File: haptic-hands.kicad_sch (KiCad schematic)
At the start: 17 parts, among them M1 Motor_DC, SW1 SW_Push_45deg

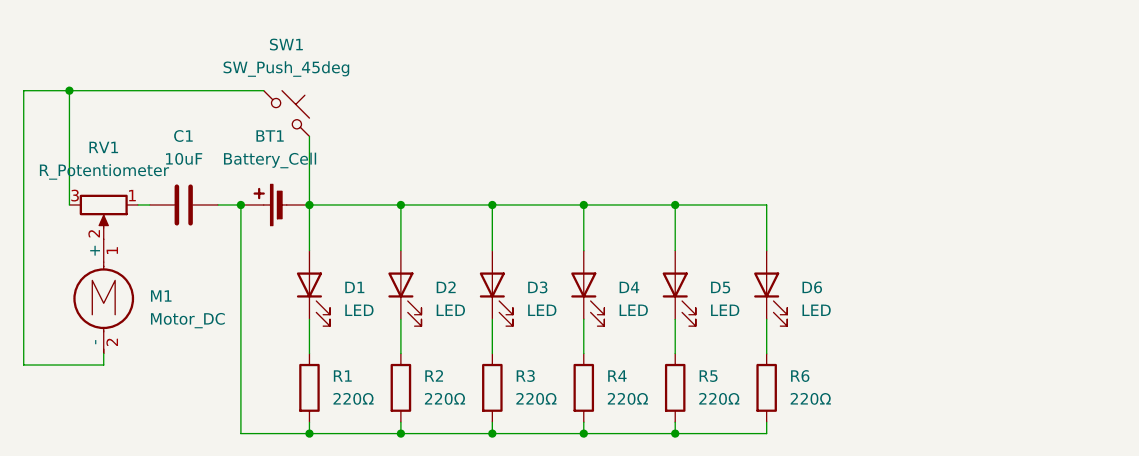
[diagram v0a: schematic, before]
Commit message: Rework schematic
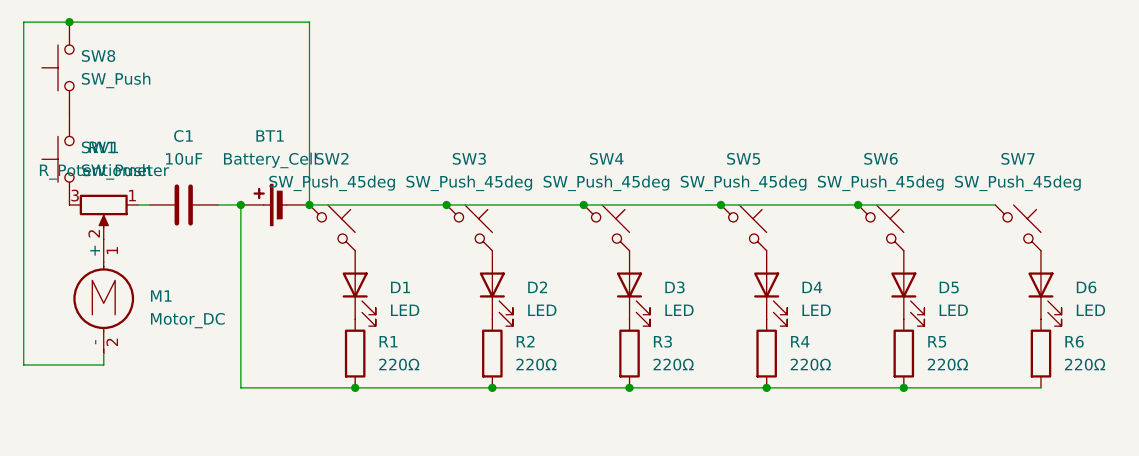
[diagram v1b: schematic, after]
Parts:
- removed SW1: SW_Push_45deg, Button_Switch_THT:SW_PUSH_6mm, symbol Switch:SW_Push_45deg
- added SW1, SW8: SW_Push, Button_Switch_THT:SW_PUSH_6mm, symbol Switch:SW_Push
- added SW2, SW3, SW4, SW5, SW6, SW7: SW_Push_45deg, Button_Switch_THT:SW_PUSH_6mm, symbol Switch:SW_Push_45deg
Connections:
- net at M1.2 (-): now also BT1.2 (-), SW2.1, SW3.1, SW4.1, SW5.1, SW6.1, SW7.1, SW8.2; no longer RV1.3
- new net: D5.2 (A), SW6.2
- new net: D1.2 (A), SW2.2
- new net: D6.2 (A), SW7.2
- new net: D3.2 (A), SW4.2
- new net: D2.2 (A), SW3.2
- new net: D4.2 (A), SW5.2
- new net: RV1.3, SW1.1
- new net: SW1.2, SW8.1

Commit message: Rework PCB
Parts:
- M1: footprint Motors:Vybronics_VZ30C1T8219732L -> Connector_PinHeader_2.54mm:PinHeader_1x02_P2.54mm_Vertical
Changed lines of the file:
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@@
 			)
 		)
-		(property "Footprint" "Motors:Vybronics_VZ30C1T8219732L"
+		(property "Footprint" "Connector_PinHeader_2.54mm:PinHeader_1x02_P2.54mm_Vertical"
 			(at 95.25 100.076 0)
 			(effects
